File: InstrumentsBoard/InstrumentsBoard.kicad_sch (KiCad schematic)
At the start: 24 parts, among them J1 RJ45_LED_Shielded, Q1 BSS138, U1 Teensy4.1_DEV-16771, U2 OKI

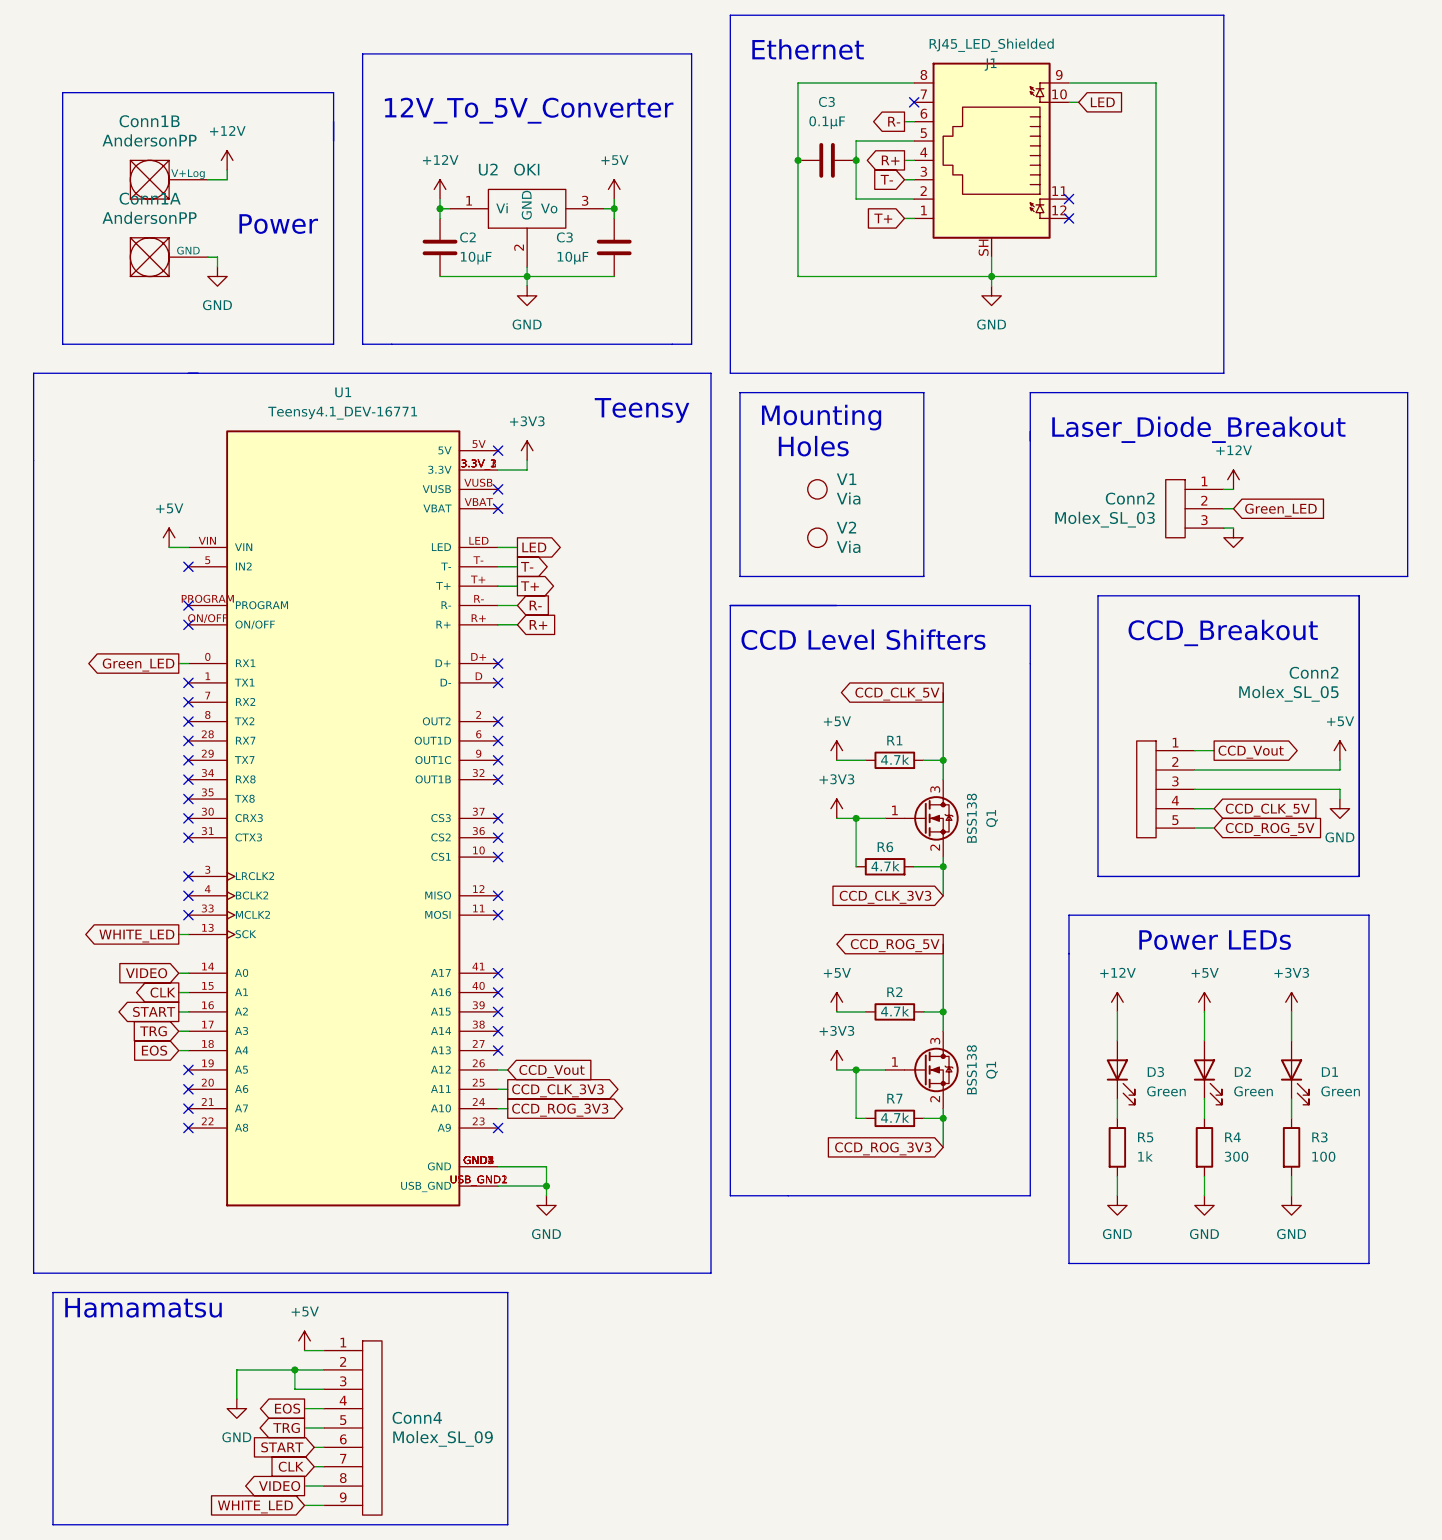
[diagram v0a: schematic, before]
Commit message: Revert "revert back to laser diode board"
This reverts commit 6528700a9c51bf2c3bc149a74fbf2f6639f4022b.
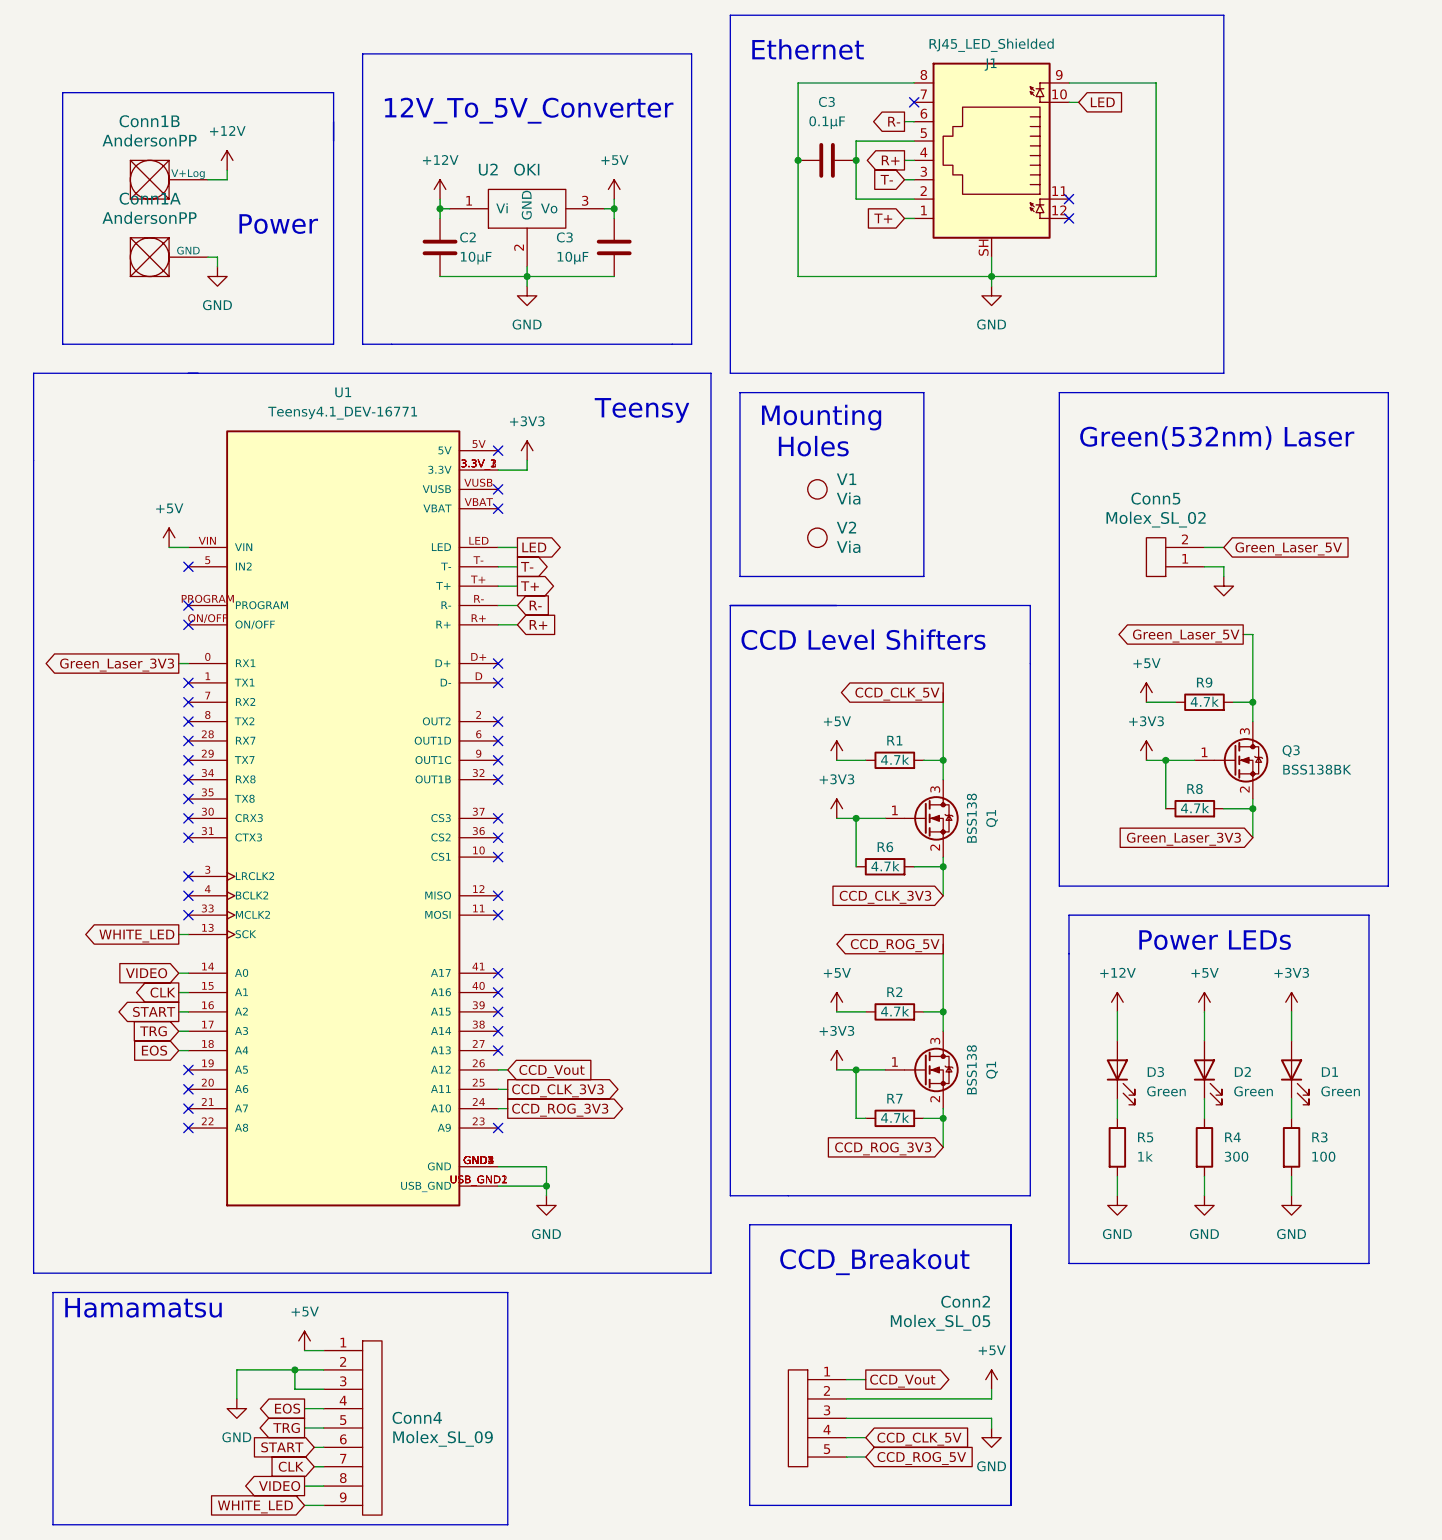
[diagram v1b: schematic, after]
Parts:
- removed Conn2: Molex_SL_03, MRDT_Connectors:MOLEX_SL_03_Vertical, symbol MRDT_Connectors:Molex_SL_03
- added Conn5: Molex_SL_02, MRDT_Connectors:MOLEX_SL_02_Vertical, symbol MRDT_Connectors:Molex_SL_02
- added Q3: BSS138BK, Package_TO_SOT_SMD:SOT-23, symbol Transistor_FET:BSS138
- added R8, R9: 4.7k, Resistor_SMD:R_0603_1608Metric_Pad0.98x0.95mm_HandSolder, symbol Device:R
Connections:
- net +3V3: now also Q3.1 (G), R8.1
- net +5V: now also R9.1
- net GND: now also Conn5.1
- net Green_LED renamed Green_Laser_3V3
- net Green_Laser_3V3: now also Q3.2 (S), R8.2
- new net Green_Laser_5V: Conn5.2, Q3.3 (D), R9.2
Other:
- note added: "Green(532nm) Laser"
- note removed: "Laser_Diode_Breakout"
- moved on the sheet: Conn2

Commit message: revert back to laser diode board
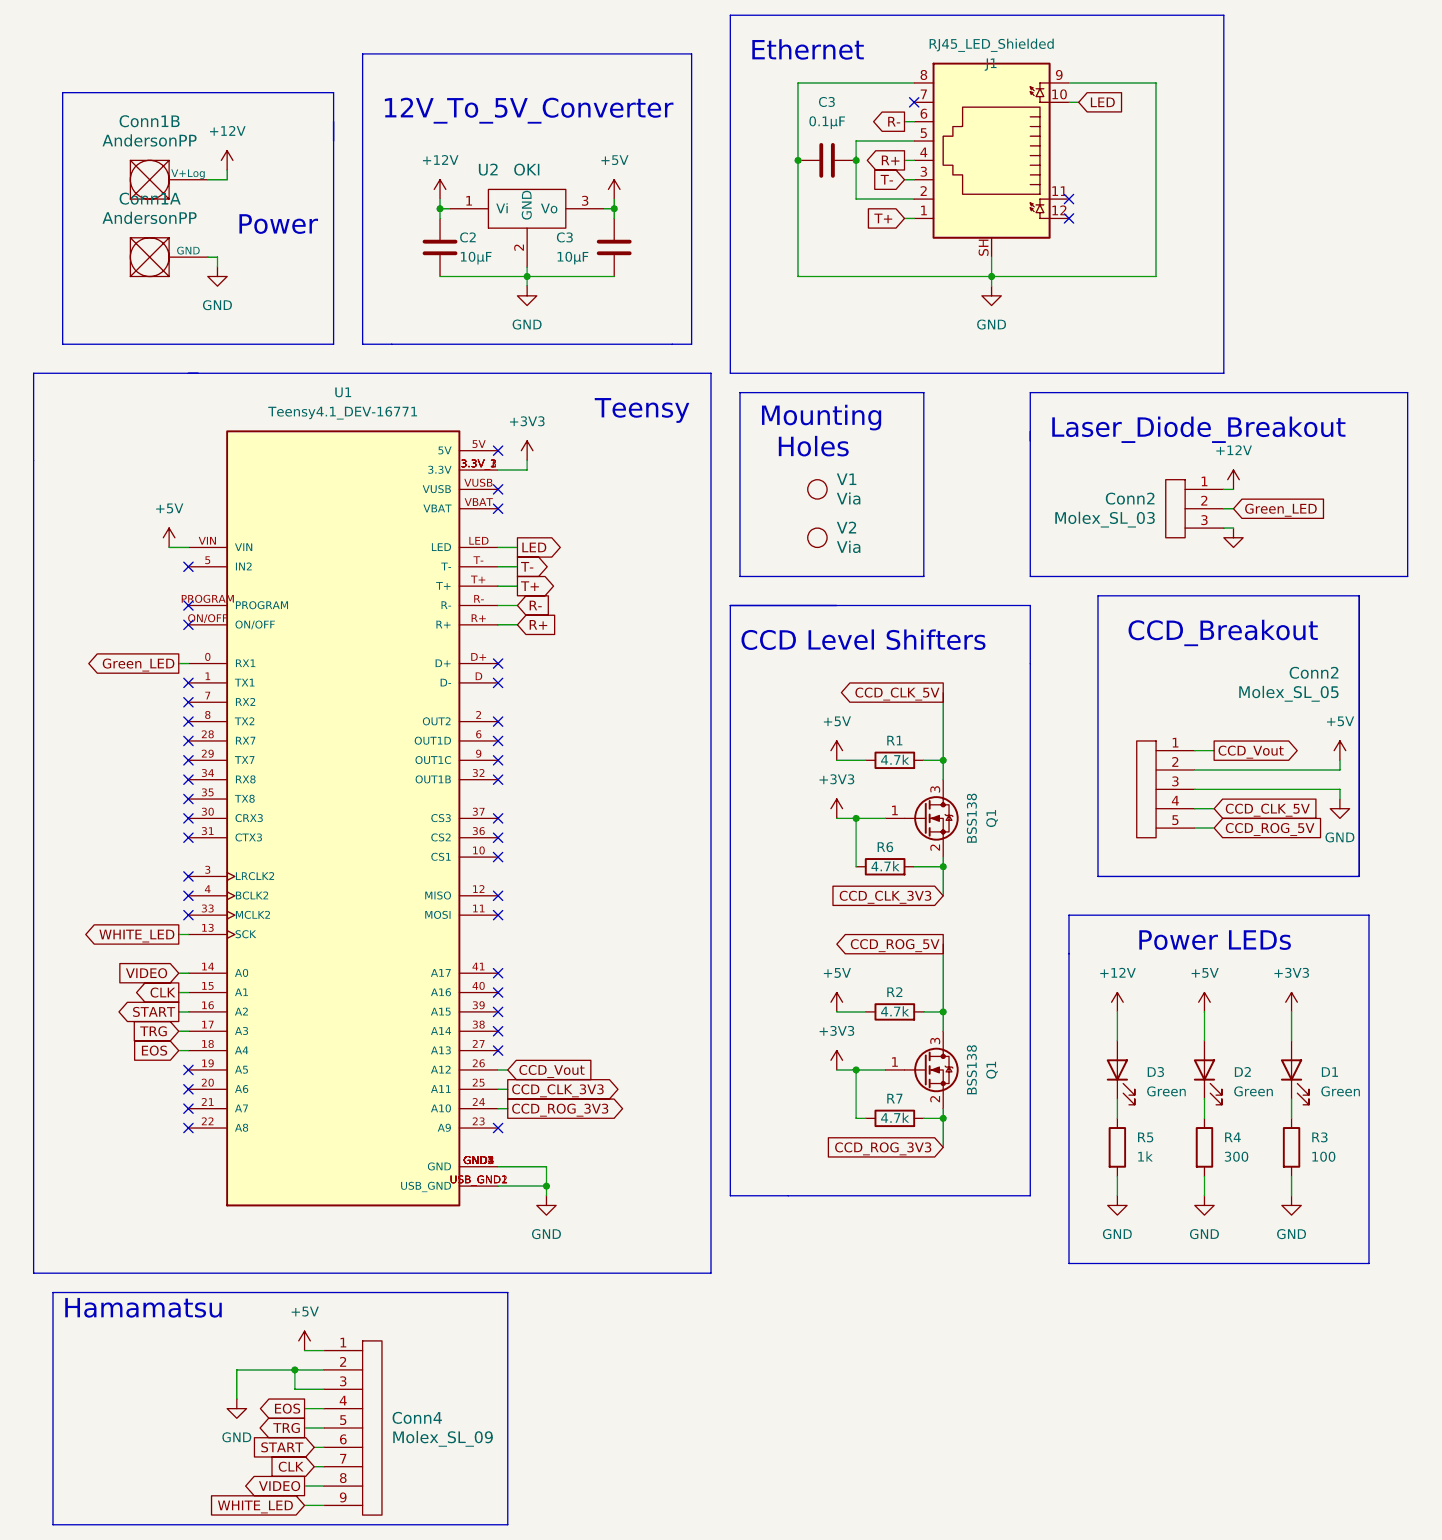
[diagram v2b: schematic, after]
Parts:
- removed Conn5: Molex_SL_02, MRDT_Connectors:MOLEX_SL_02_Vertical, symbol MRDT_Connectors:Molex_SL_02
- removed Q3: BSS138BK, Package_TO_SOT_SMD:SOT-23, symbol Transistor_FET:BSS138
- removed R8, R9: 4.7k, Resistor_SMD:R_0603_1608Metric_Pad0.98x0.95mm_HandSolder, symbol Device:R
- added Conn2: Molex_SL_03, MRDT_Connectors:MOLEX_SL_03_Vertical, symbol MRDT_Connectors:Molex_SL_03
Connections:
- net +12V: now also Conn2.1
- net GND: now also Conn2.3
- net Green_Laser_3V3 renamed Green_LED
- net Green_LED: now also Conn2.2
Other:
- note added: "Laser_Diode_Breakout"
- note removed: "Green(532nm) Laser"
- moved on the sheet: Conn2
